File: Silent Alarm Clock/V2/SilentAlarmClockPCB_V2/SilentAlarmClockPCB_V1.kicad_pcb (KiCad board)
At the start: 4 copper layers, 52 x 31 mm, 28 parts, among them J1 USB_C_Receptacle_USB2.0_16P, J2 Barrel_Jack, J3 B2B-PH-K-S, SW3 RESET, SW4 BOOT, U1 ESD7104MUTAG, U2 ESP32-S3-MINI-1-N8, U3 BQ24040DSQR, U4 TLV75801PDRV

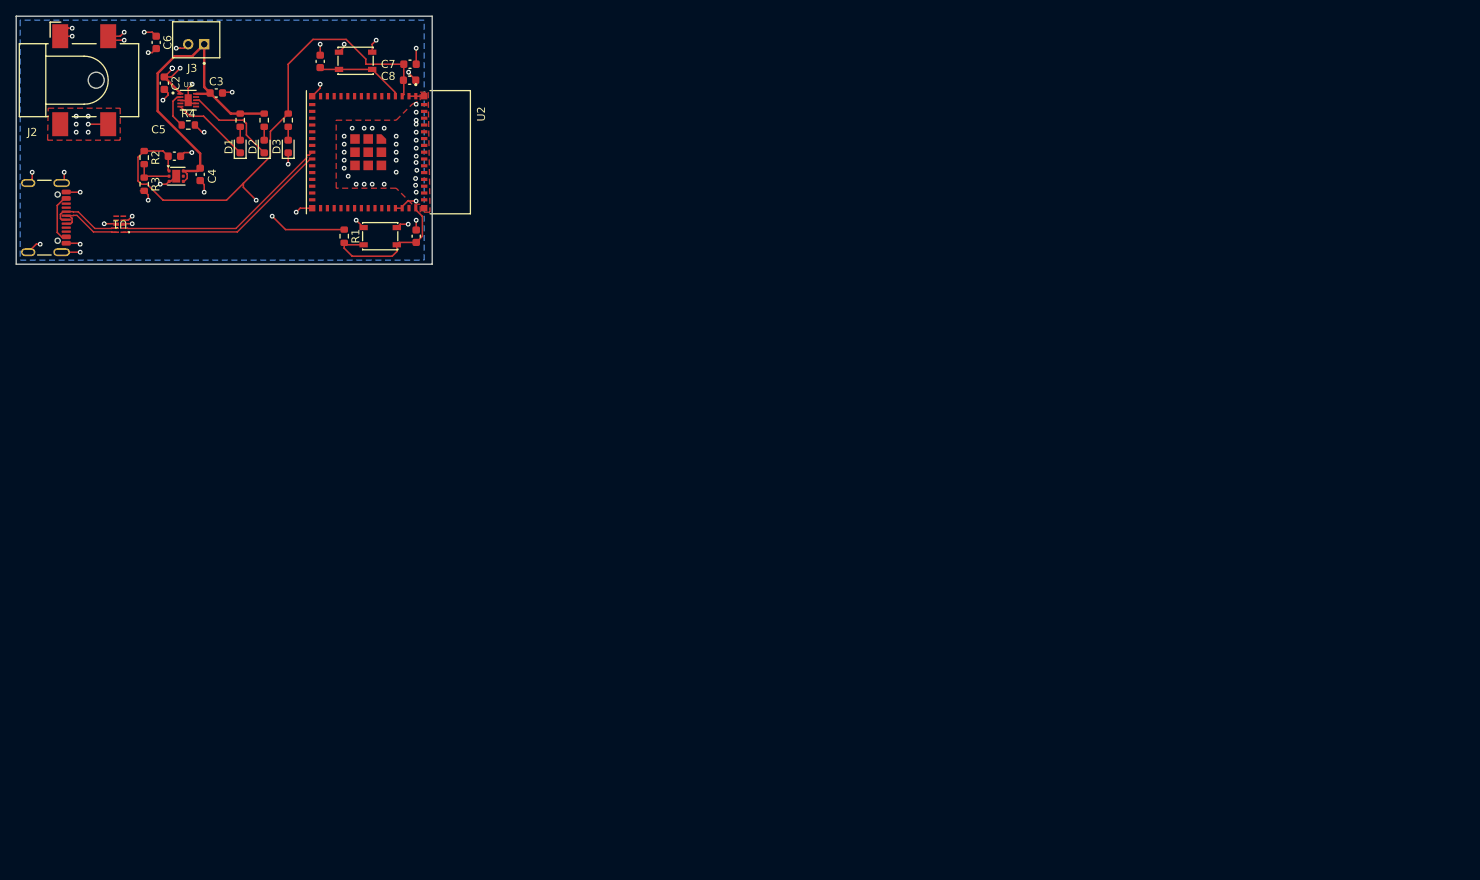
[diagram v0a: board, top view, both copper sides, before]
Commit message: V2 preliminary layout
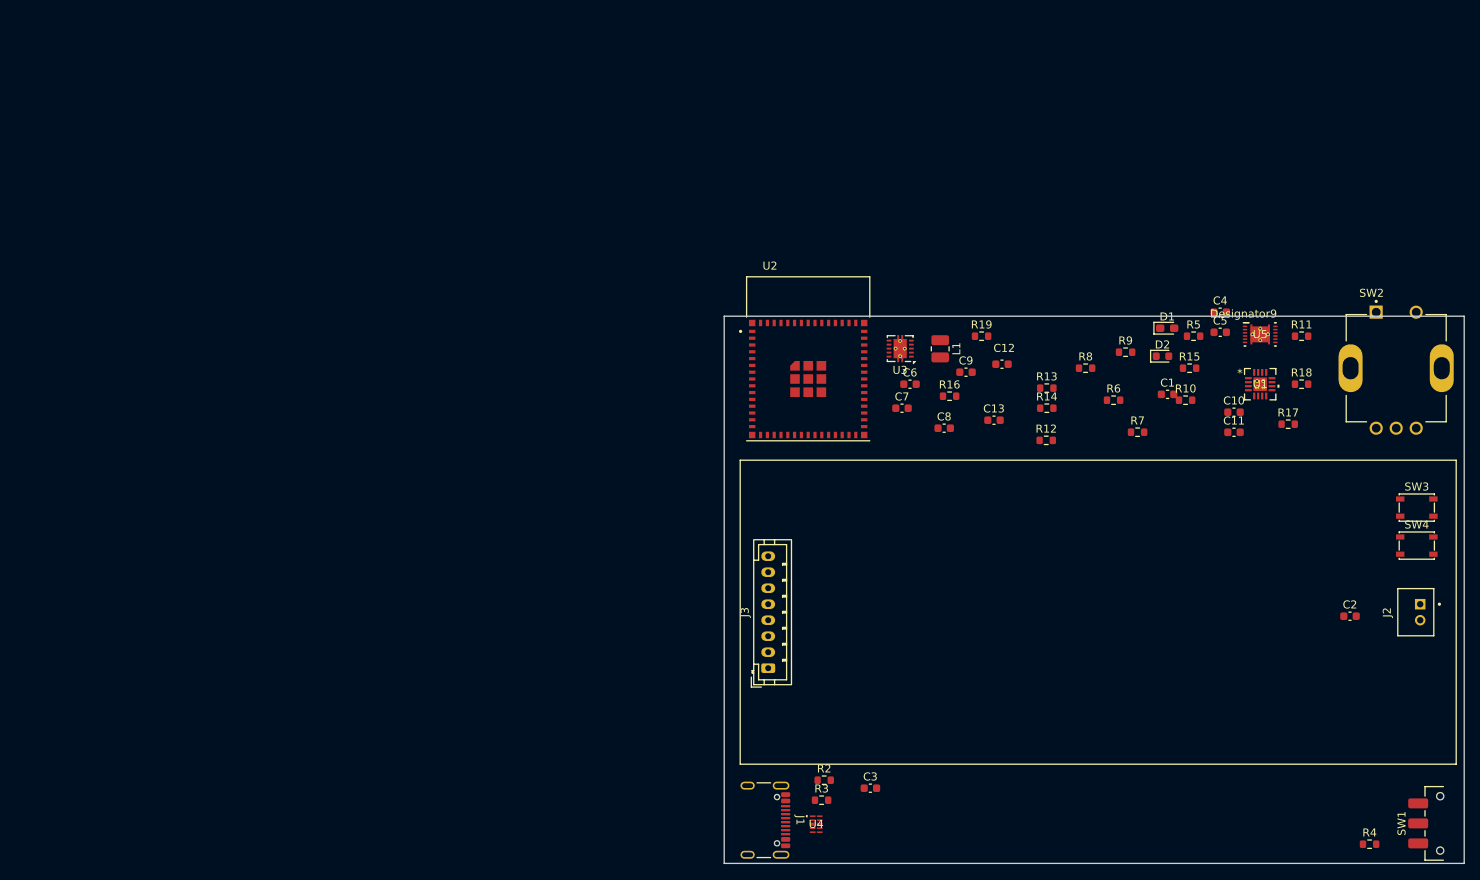
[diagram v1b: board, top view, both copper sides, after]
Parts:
- removed D3: LED, LED_SMD:LED_0603_1608Metric
- removed R1: 1k, Resistor_SMD:R_0603_1608Metric
- added C1: 10uF, Capacitor_SMD:C_0603_1608Metric, F.Cu at (170.4, 76.3)
- added C11: 1uF, Capacitor_SMD:C_0603_1608Metric, F.Cu at (178.7, 81.0)
- added C12: 0.1uF, Capacitor_SMD:C_0603_1608Metric, F.Cu at (149.7, 72.5)
- added C13: 0.1uF, Capacitor_SMD:C_0603_1608Metric, F.Cu at (148.7, 79.5)
- added L1: 2.2uH, Inductor_SMD:L_1008_2520Metric, F.Cu at (142.0, 70.6)
- added R10: 100k, Resistor_SMD:R_0603_1608Metric, F.Cu at (172.7, 77.0)
- added R11: 0.01, Resistor_SMD:R_0603_1608Metric, F.Cu at (187.2, 69.0)
- added R12: 4.7k, Resistor_SMD:R_0603_1608Metric, F.Cu at (155.3, 82.0)
- added R13: 4.7k, Resistor_SMD:R_0603_1608Metric, F.Cu at (155.3, 75.5)
- added R14: 10k, Resistor_SMD:R_0603_1608Metric, F.Cu at (155.3, 78.0)
- added R15: 10k, Resistor_SMD:R_0603_1608Metric, F.Cu at (173.2, 73.0)
- added R16: 10k, Resistor_SMD:R_0603_1608Metric, F.Cu at (143.2, 76.5)
- added R17: 10k, Resistor_SMD:R_0603_1608Metric, F.Cu at (185.5, 80.0)
- added R18: 10k, Resistor_SMD:R_0603_1608Metric, F.Cu at (187.2, 75.0)
- added R19: 10k, Resistor_SMD:R_0603_1608Metric, F.Cu at (147.2, 69.0)
- added R8: 180, Resistor_SMD:R_0603_1608Metric, F.Cu at (160.2, 73.0)
- added R9: 1k, Resistor_SMD:R_0603_1608Metric, F.Cu at (165.2, 71.0)
- added SW1: SW_SPDT, Button_Switch_SMD:SW_SPDT_CK_JS102011SAQN, F.Cu at (204.5, 129.9)
- added SW2: RotaryEncoder_Switch, PEC11R_4220F_S0024:XDCR_PEC11R-4220F-S0024, F.Cu at (199.0, 73.0)
- added U5: BQ27441DRZT-G1A, BQ27441DRZT-G1A:Copy of DRZ0012A, F.Cu at (182.0, 68.8)
- C10, C9: value 0.1uF -> 1uF
- C3: value 1uF -> 10uF
- C5: value 1uF -> 0.47uF
- C6, C7, C8: value C -> 1uF
- D1: footprint LED_SMD:LED_0603_1608Metric -> LED_SMD:LED_0603_1608Metric_Pad1.05x0.95mm_HandSolder
- J2: value Barrel_Jack -> B2B-PH-K-S; footprint Connector_BarrelJack:BarrelJack_CLIFF_FC681465S_SMT_Horizontal -> B2B-PH-K-S:JST_B2B-PH-K-S
- J3: value B2B-PH-K-S -> Conn_01x08_Socket; footprint B2B_PH_K_S:JST_B2B-PH-K-S -> Connector_JST:JST_PH_B8B-PH-K_1x08_P2.00mm_Vertical
- R2, R3: value R -> 5.1k
- R4: value 540 -> 100k
- R5: value 1k -> 10k
- R6: value 1k -> 590
- R7: value 1k -> 440
- U1: value ESD7104MUTAG -> BQ24075TRGTR; footprint ESD7104MUTAG:UDFN10_ONS -> BQ24075TRGTR:RGT16_1P7X1P7
- U3: value BQ24040DSQR -> TPS63001; footprint BQ24040DSQR:SON40P200X200X80-11N -> Package_SON:Texas_DRC0010J_ThermalVias
- U4: value TLV75801PDRV -> ESD7104MUTAG; footprint Package_SON:WSON-6-1EP_2x2mm_P0.65mm_EP1x1.6mm -> ESD7104MUTAG:UDFN10_ONS
- moved J2 179.2 mm to (201.4, 103.5), turned to 90 degrees
- moved R4 172.9 mm to (195.7, 132.5)
- moved C2 162.5 mm to (193.2, 104.0), turned to 0 degrees
- moved SW4 145.8 mm to (201.6, 95.2)
- moved U1 144.0 mm to (182.0, 75.0), turned to 0 degrees
- moved SW3 133.9 mm to (201.6, 90.4)
- moved C5 132.6 mm to (177.0, 68.5)
- moved C4 128.7 mm to (177.0, 66.0), turned to 0 degrees
- moved C10 122.4 mm to (178.7, 78.5), turned to 0 degrees
- moved R5 122.2 mm to (173.7, 69.0), turned to 0 degrees
- moved C3 119.3 mm to (133.3, 125.5)
- moved D1 118.1 mm to (170.4, 68.0), turned to 0 degrees
- moved J1 117.3 mm to (119.0, 129.5)
- moved D2 115.3 mm to (169.8, 71.5), turned to 0 degrees
- moved R2 115.2 mm to (127.5, 124.5), turned to 0 degrees
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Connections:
- C10 pad 1: Net-(U2-IO0) -> GND
- C10 pad 2: GND -> Encoder_A
- C2 pad 1: /5VIN -> BATTERY_IN
- C3 pad 1: Net-(U3-OUT) -> V_USB
- C4 pad 1: Net-(U3-OUT) -> GND
- C4 pad 2: GND -> BATTERY_IN
- C5 pad 1: /3V3 -> GND
- C5 pad 2: GND -> 1.8V
- C6 pad 1: /5VIN -> GND
- C6 pad 2: GND -> OUT
- C7 pad 1: /3V3 -> GND
- C7 pad 2: GND -> Net-(U3-EN)
- C8 pad 1: /3V3 -> GND
- C8 pad 2: GND -> 3V3
- C9 pad 1: Net-(U2-EN) -> GND
- C9 pad 2: GND -> 3V3
- D1 pad 2: Net-(D1-A) -> OUT
- D2 pad 2: Net-(D2-A) -> OUT
- J1 pad A4: Net-(J1-VBUS-PadA4) -> V_USB
- J1 pad A5: unconnected-(J1-CC1-PadA5) -> CC1
- J1 pad A6: /USB_P -> D+
- J1 pad A7: /USB_N -> D-
- J1 pad A9: Net-(J1-VBUS-PadA4) -> V_USB
- J1 pad B4: Net-(J1-VBUS-PadA4) -> V_USB
- J1 pad B5: unconnected-(J1-CC2-PadB5) -> CC2
- J1 pad B6: /USB_P -> D+
- J1 pad B7: /USB_N -> D-
- J1 pad B9: Net-(J1-VBUS-PadA4) -> V_USB
- J1 pad SH: GND -> SHEILD
- J2 pad 1: /5VIN -> GND
- J2 pad 2: GND -> BATTERY_IN
- J3 pad 1: Net-(U3-OUT) -> 3V3
- R2 pad 1: /3V3 -> CC1
- R2 pad 2: Net-(U4-FB) -> GND
- R3 pad 1: Net-(U4-FB) -> CC2
- R4 pad 1: Net-(U3-ISET) -> Net-(SW1-A)
- R4 pad 2: GND -> BATTERY_IN
- R5 pad 1: Net-(U3-OUT) -> GND
- R5 pad 2: Net-(D1-A) -> Net-(U1-TS)
- R6 pad 1: Net-(U3-OUT) -> Net-(U1-ISET)
- R6 pad 2: Net-(D2-A) -> GND
- R7 pad 1: /3V3 -> Net-(U1-ILIM)
- R7 pad 2: Net-(D3-A) -> GND
- U1 pad 1: /USB_P -> Net-(U1-TS)
- U1 pad 10: unconnected-(U1-NC-Pad10) -> OUT
- U1 pad 2: /USB_N -> BATTERY_IN
- U1 pad 3: GND -> BATTERY_IN
- U1 pad 4: /5VIN -> Net-(U1-*CE)
- U1 pad 5: unconnected-(U1-I/O-Pad5) -> GND
- U1 pad 6: unconnected-(U1-NC-Pad6) -> Net-(U1-EN1)
- U1 pad 7: unconnected-(U1-NC-Pad7) -> PGOOD
- U1 pad 9: unconnected-(U1-NC-Pad9) -> Net-(U1-*CHG)
- U2 pad 12: unconnected-(U2-IO8-Pad12) -> SDA
- U2 pad 13: unconnected-(U2-IO9-Pad13) -> SCL
- U2 pad 14: unconnected-(U2-IO10-Pad14) -> CS
- U2 pad 15: unconnected-(U2-IO11-Pad15) -> DIN
- U2 pad 16: unconnected-(U2-IO12-Pad16) -> CLK
- U2 pad 17: unconnected-(U2-IO13-Pad17) -> D/C
- U2 pad 18: unconnected-(U2-IO14-Pad18) -> RST
- U2 pad 19: unconnected-(U2-IO15-Pad19) -> BUSY
- U2 pad 23: /USB_N -> D-
- U2 pad 24: /USB_P -> D+
- U2 pad 25: unconnected-(U2-IO21-Pad25) -> S1
- U2 pad 28: unconnected-(U2-IO33-Pad28) -> Encoder_A
- U2 pad 29: unconnected-(U2-IO34-Pad29) -> Encoder_B
- U2 pad 3: /3V3 -> 3V3
- U3 pad 1: /5VIN -> 3V3
- U3 pad 10: Net-(U3-OUT) -> 3V3
- U3 pad 2: Net-(U3-ISET) -> Net-(U3-L2)
- U3 pad 4: unconnected-(U3-PRETERM-Pad4) -> Net-(U3-L1)
- U3 pad 5: Net-(D1-K) -> OUT
- U3 pad 6: (no net) -> Net-(U3-EN)
- U3 pad 7: GND -> Net-(U3-EN)
- U3 pad 8: Net-(D2-K) -> Net-(U3-EN)
- U3 pad 9: unconnected-(U3-TS-Pad9) -> GND
- U4 pad 1: /3V3 -> D-
- U4 pad 2: Net-(U4-FB) -> D+
- U4 pad 4: Net-(U3-OUT) -> V_USB
- U4 pad 6: Net-(U3-OUT) -> unconnected-(U4-NC-Pad6)
- U4 pad 7: GND -> unconnected-(U4-NC-Pad7)
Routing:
- net /3V3: track 78.3 -> 0.00 mm, vias 2 -> 0
- net GND: track 58.2 -> 0.00 mm, vias 68 -> 0
- net Net-(U3-OUT): track 41.5 -> 0.00 mm
- net /5VIN: track 40.1 -> 0.00 mm, vias 10 -> 0
- net /USB_N: track 37.1 -> 0.00 mm
- net /USB_P: track 36.7 -> 0.00 mm
- net Net-(U2-EN): track 18.8 -> 0.00 mm
- net Net-(D2-K): track 12.1 -> 0.00 mm
- net Net-(U2-IO0): track 11.1 -> 0.00 mm
- net Net-(D1-K): track 9.88 -> 0.00 mm
- net Net-(J1-VBUS-PadA4): track 6.21 -> 0.00 mm
- net Net-(U4-FB): track 4.86 -> 0.00 mm
- net Net-(U3-ISET): track 4.54 -> 0.00 mm
- net Net-(D3-A): track 1.67 -> 0.00 mm
- net Net-(D2-A): track 1.67 -> 0.00 mm
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- removed copper zone on In2.Cu, net /5VIN
- removed copper zone on B.Cu, net GND
- removed copper zone on F.Cu, net GND
- removed copper zone on In1.Cu, net GND
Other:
- board size 52 x 31 mm -> 92.5 x 68.4 mm
